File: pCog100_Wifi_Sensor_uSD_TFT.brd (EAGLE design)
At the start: 48 x 28 mm, 31 parts

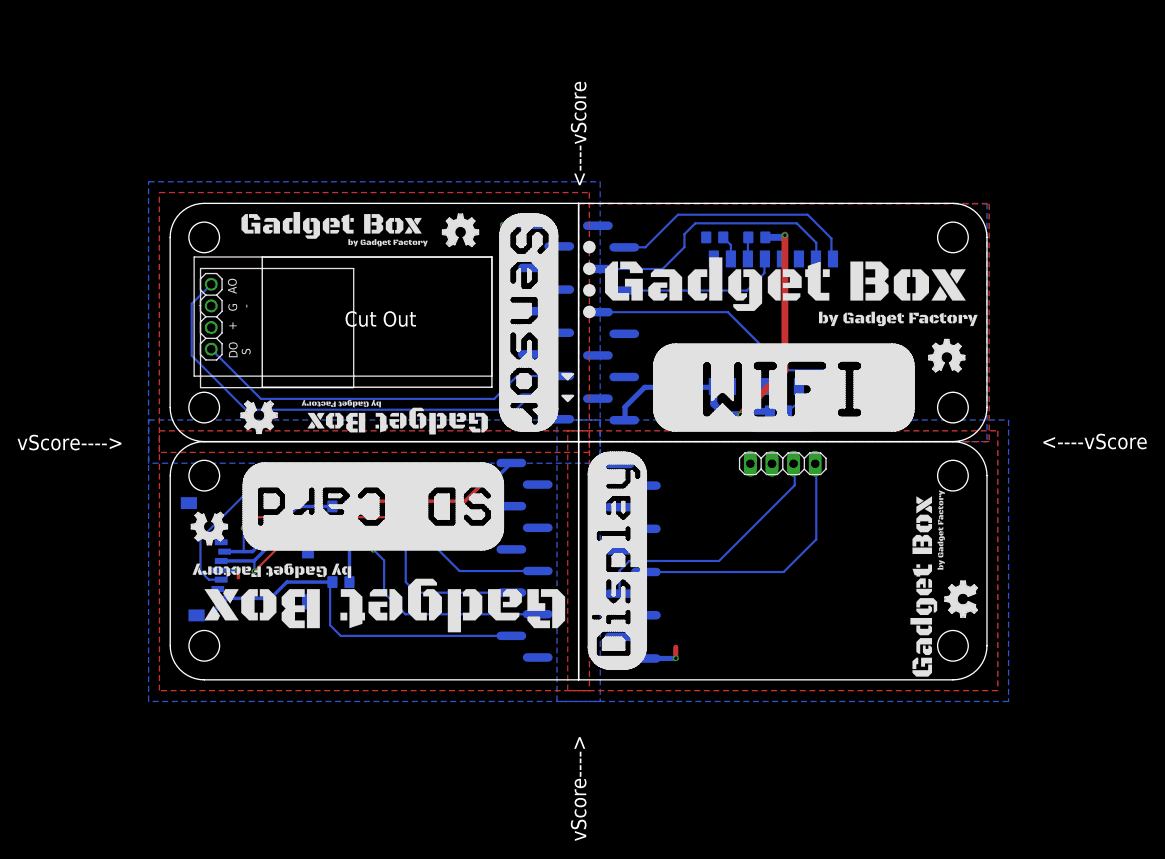
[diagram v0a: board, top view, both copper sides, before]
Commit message: All the 2.0 updates
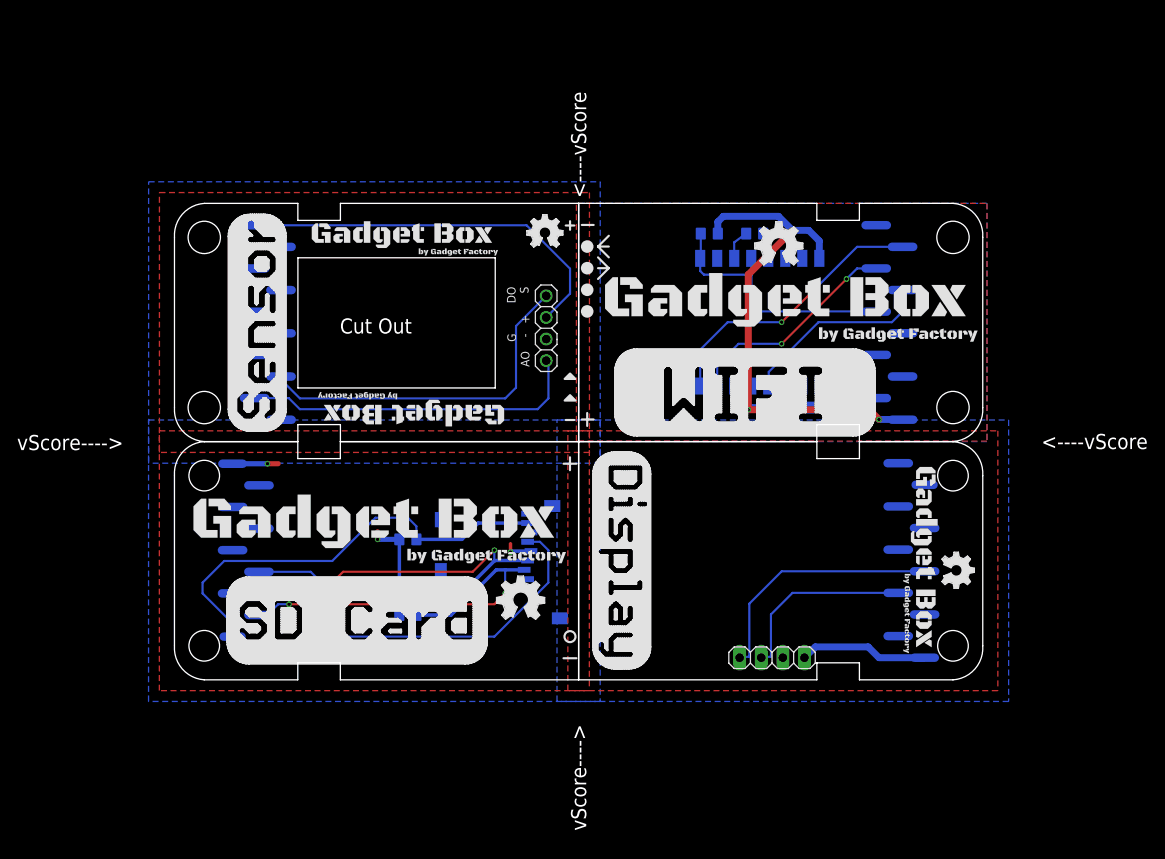
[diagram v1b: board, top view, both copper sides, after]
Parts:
- removed U$17: (no value), ohw-logo:OSHW_FILLX150_NOTEXT
- ECOG: value ECOG_GENERAL_ROWECOG_GENERAL_SMD -> ECOG_BUSES_ROWECOG_BUSES_SMD; device eCogs:ECOG_GENERAL_SMD -> eCogs:ECOG_BUSES_SMD
- ECOG3: value ECOG_BUSES_ROWECOG_BUSES_SMD -> ECOG_GENERAL_ROWECOG_GENERAL_SMD; device eCogs:ECOG_BUSES_SMD -> eCogs:ECOG_GENERAL_SMD
- R1, R2, R3: value 10K -> 47K; device GadgetFactory:0805 -> GadgetFactory_6.0:0805
- R5, R6, R7: value 47K -> 10K; device GadgetFactory_6.0:0805 -> GadgetFactory:0805
- U$10: device GadgetFactory:GADGETBOX_TEXT -> GadgetFactory:GADGETBOX_SMALL
- U$11: device GadgetFactory:GADGETBOX_SMALL -> GadgetFactory:GADGETBOX_TEXT
- U$12: device GadgetFactory:GADGETBOX_SMALL -> eCogs:LEGEND_DIO
- U$13, U$14, U$15: device ohw-logo:OSHW_FILLX150_NOTEXT -> eCogs:LEGEND_DIO
- U$16: device ohw-logo:OSHW_FILLX150_NOTEXT -> ohw-logo:OSHW_FILLX200_NOTEXT
- U$2: device eCogs:LEGEND_DIO -> ohw-logo:OSHW_FILLX200_NOTEXT
- U$3: device eCogs:LEGEND_DIO -> GadgetFactory:GADGETBOX_SMALL
- U$4: device eCogs:LEGEND_DIO -> ohw-logo:OSHW_FILLX150_NOTEXT
- U$5: value (none) -> SENSOR; device eCogs:LEGEND_DIO -> eCogs:SENSOR-HJX4
- U$6: device GadgetFactory:GADGETBOX_SMALL -> eCogs:LEGEND_ANALOG
- U$7: value SENSOR -> (none); device eCogs:SENSOR-HJX4 -> eCogs:LEGEND_ANALOG
- U$8: device eCogs:LEGEND_ANALOG -> GadgetFactory:GADGETBOX_SMALL
- U$9: device eCogs:LEGEND_ANALOG -> ohw-logo:OSHW_FILLX150_NOTEXT
- moved U$14 61.5 mm to (49.0, 48.4), turned to 180 degrees
- moved R5 59.8 mm to (76.2, 32.0), turned to 0 degrees
- moved R7 58.3 mm to (68.7, 52.4)
- moved U$1 55.8 mm to (24.0, 18.4)
- moved ECOG1 55.6 mm to (96.0, 28.0), turned to 180 degrees
- moved ECOG 55.6 mm to (0.00, 0.00)
- moved ECOG3 55.6 mm to (96.0, 56.0)
- moved ECOG2 55.6 mm to (0.01, 28.0), turned to 0 degrees
- moved R6 55.4 mm to (63.4, 52.4)
- moved R2 55.2 mm to (27.9, 10.2), turned to 0 degrees
- moved R3 54.4 mm to (27.9, 7.62)
- moved R1 54.2 mm to (27.9, 16.5), turned to 0 degrees
- moved U$15 52.6 mm to (49.0, 50.9)
- moved U$3 51.9 mm to (88.6, 14.4), turned to 270 degrees
- moved U$4 51.6 mm to (90.7, 15.0), turned to 270 degrees
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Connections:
- removed net RX: ECOG.G1, X1.15
- removed net TX: ECOG.G0, X1.16
- new net RX/MOSI: ECOG3.G1, X1.15
- new net TX/MISO: ECOG3.G0, X1.16
- net 3V3: now also R2.2, U$5.+; no longer R5.2, U$7.+
- net A1: now also U$5.AO; no longer U$7.AO
- net A2: now also U$5.DO/S; no longer U$7.DO/S
- net GND: now also R5.1, U$5.GND; no longer R2.1, U$7.GND
- net GPIO0/BOOTLOAD: now also ECOG3.G2; no longer ECOG.G2
- net N$3: now also R4.1; no longer R1.1
- net N$4: now also R5.2; no longer R2.2
- net N$5: now also R7.1; no longer R4.1
- net RESET: now also ECOG3.G3, R6.1; no longer ECOG.G3, R3.1
- net SD_!CS: now also ECOG.SPI-CS, R3.1; no longer ECOG3.SPI-CS, R7.1
- net SD_MISO: now also ECOG.SPI-MISO, R1.1; no longer ECOG3.SPI-MISO, R5.1
- net SD_MOSI: now also ECOG.SPI-MOSI, R2.1; no longer ECOG3.SPI-MOSI, R6.1
- net SD_SCK: now also ECOG.SPI-SCK; no longer ECOG3.SPI-SCK
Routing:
- net 3V3: track 102.2 -> 147.2 mm, vias 7 -> 6
- net TX/MISO: track 0.00 -> 33.3 mm, vias 0 -> 2
- net RX: track 31.6 -> 0.00 mm
- net TX: track 29.6 -> 0.00 mm
- net RX/MOSI: track 0.00 -> 25.9 mm, vias 0 -> 2
- net A1: track 52.6 -> 40.1 mm
- net SD_MISO: track 40.9 -> 52.3 mm
- net SD_MOSI: track 55.7 -> 46.8 mm
- net SD_SCK: track 57.0 -> 48.5 mm
- net N$1: track 30.0 -> 22.1 mm
- net SD_!CS: track 55.3 -> 48.7 mm
- net RESET: track 37.3 -> 30.9 mm
- net GPIO0/BOOTLOAD: track 19.0 -> 22.9 mm
- net A2: track 44.4 -> 41.7 mm
- net N$2: track 30.6 -> 29.5 mm
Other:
- board size 48 x 28 mm -> 47.5 x 28 mm
- board text added: "0"
- board text added: "1"
- board text added: "2"
- board text added: "3"
- board text added: "RX/MOSI"
- board text added: "SPI-CS"
- board text added: "SPI-MISO"
- board text added: "SPI-MOSI"
- board text added: "SPI-SCK"
- board text added: "TX/MISO"
- board text added: "ecog100 v2.0"
- board text added: "ecog101 v2.0"
- board text added: "ecog102 v2.0"
- board text added: "ecog103 v2.0"
- board text removed: "RX>"
- board text removed: "SPI-CS>"
- board text removed: "SPI-MISO>"
- board text removed: "SPI-MOSI<"
- board text removed: "SPI-SCK>"
- board text removed: "TX<"
- board text removed: "ecog100 v1.1"
- board text removed: "ecog101 v1.1"
- board text removed: "ecog102 v1.1"
- board text removed: "ecog103 v1.2"
